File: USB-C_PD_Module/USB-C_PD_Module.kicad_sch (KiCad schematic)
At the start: 0 parts

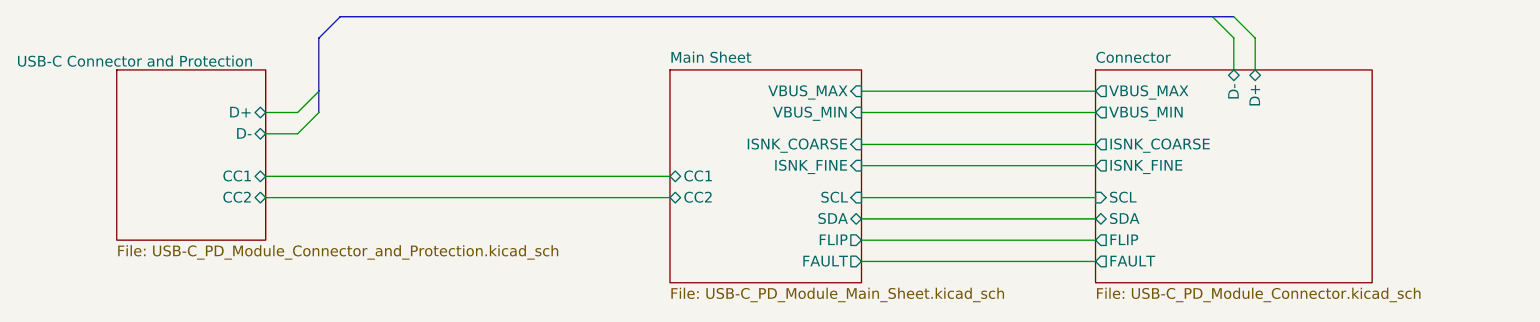
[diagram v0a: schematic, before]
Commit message: Module Basics
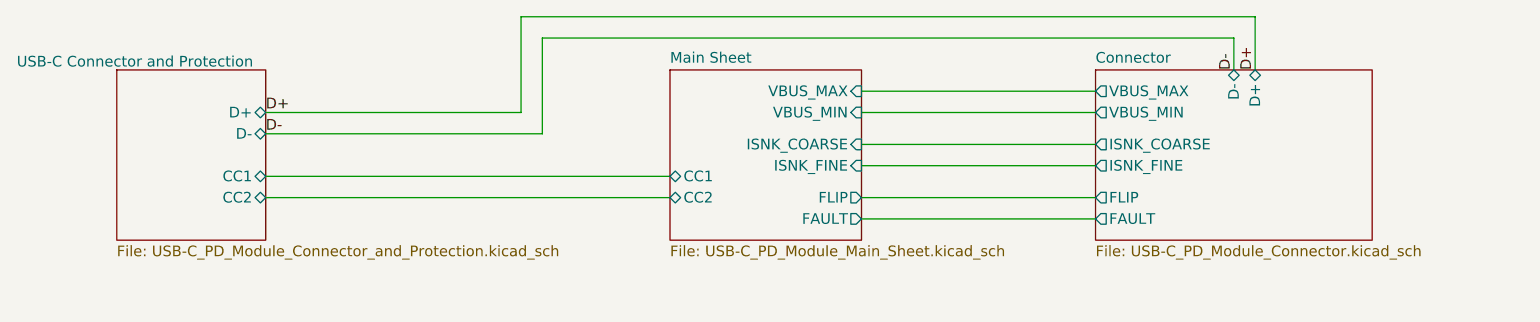
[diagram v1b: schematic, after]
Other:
- sheet Connector ports: added none; removed SCL, SDA
- sheet Main Sheet ports: added none; removed SCL, SDA
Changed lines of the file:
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@@
 		(rev "1.0")
 	)
-	(bus_entry
-		(at 210.82 88.9)
-		(size 2.54 2.54)
-		(stroke
-			(width 0)
-			(type default)
-		)
-	)
-	(bus_entry
-		(at 101.6 102.87)
-		(size 2.54 -2.54)
-		(stroke
-			(width 0)
-			(type default)
-		)
-	)
-	(bus_entry
-		(at 213.36 88.9)
-		(size 2.54 2.54)
-		(stroke
-			(width 0)
-			(type default)
-		)
-	)
-	(bus_entry
-		(at 101.6 100.33)
-		(size 2.54 -2.54)
-		(stroke
-			(width 0)
-			(type default)
-		)
-	)
 	(wire
 		(pts
@@
 	(wire
 		(pts
+			(xy 168.91 97.79) (xy 196.85 97.79)
+		)
+		(stroke
+			(width 0)
+			(type default)
+		)
+	)
+	(wire
+		(pts
+			(xy 215.9 88.9) (xy 215.9 95.25)
+		)
+		(stroke
+			(width 0)
+			(type default)
+		)
+	)
+	(wire
+		(pts
+			(xy 130.81 102.87) (xy 130.81 91.44)
+		)
+		(stroke
+			(width 0)
+			(type default)
+		)
+	)
+	(wire
+		(pts
+			(xy 168.91 106.68) (xy 196.85 106.68)
+		)
+		(stroke
+			(width 0)
+			(type default)
+		)
+	)
+	(wire
+		(pts
+			(xy 168.91 100.33) (xy 196.85 100.33)
+		)
+		(stroke
+			(width 0)
+			(type default)
+		)
+	)
+	(wire
+		(pts
+			(xy 128.27 88.9) (xy 215.9 88.9)
+		)
+		(stroke
+			(width 0)
+			(type default)
+		)
+	)
+	(wire
+		(pts
+			(xy 168.91 110.49) (xy 196.85 110.49)
+		)
+		(stroke
+			(width 0)
+			(type default)
+		)
+	)
+	(wire
+		(pts
 			(xy 168.91 113.03) (xy 196.85 113.03)
 		)
@@
 	(wire
 		(pts
-			(xy 168.91 97.79) (xy 196.85 97.79)
-		)
-		(stroke
-			(width 0)
-			(type default)
-		)
-	)
-	(wire
-		(pts
-			(xy 215.9 91.44) (xy 215.9 95.25)
-		)
-		(stroke
-			(width 0)
-			(type default)
-		)
-	)
-	(bus
-		(pts
-			(xy 104.14 91.44) (xy 106.68 88.9)
-		)
-		(stroke
-			(width 0)
-			(type default)
-		)
-	)
-	(wire
-		(pts
-			(xy 168.91 110.49) (xy 196.85 110.49)
-		)
-		(stroke
-			(width 0)
-			(type default)
-		)
-	)
-	(wire
-		(pts
-			(xy 168.91 106.68) (xy 196.85 106.68)
-		)
-		(stroke
-			(width 0)
-			(type default)
-		)
-	)
-	(wire
-		(pts
-			(xy 168.91 100.33) (xy 196.85 100.33)
-		)
-		(stroke
-			(width 0)
-			(type default)
-		)
-	)
-	(bus
-		(pts
-			(xy 104.14 97.79) (xy 104.14 100.33)
-		)
-		(stroke
-			(width 0)
-			(type default)
-		)
-	)
-	(wire
-		(pts
-			(xy 168.91 115.57) (xy 196.85 115.57)
-		)
-		(stroke
-			(width 0)
-			(type default)
-		)
-	)
-	(wire
-		(pts
-			(xy 168.91 118.11) (xy 196.85 118.11)
-		)
-		(stroke
-			(width 0)
-			(type default)
-		)
-	)
-	(bus
-		(pts
-			(xy 210.82 88.9) (xy 213.36 88.9)
-		)
-		(stroke
-			(width 0)
-			(type default)
-		)
-	)
-	(wire
-		(pts
 			(xy 97.79 107.95) (xy 146.05 107.95)
 		)
@@
 	(wire
 		(pts
-			(xy 97.79 102.87) (xy 101.6 102.87)
-		)
-		(stroke
-			(width 0)
-			(type default)
-		)
-	)
-	(wire
-		(pts
-			(xy 97.79 100.33) (xy 101.6 100.33)
-		)
-		(stroke
-			(width 0)
-			(type default)
-		)
-	)
-	(bus
-		(pts
-			(xy 104.14 91.44) (xy 104.14 97.79)
-		)
-		(stroke
-			(width 0)
-			(type default)
-		)
-	)
-	(bus
-		(pts
-			(xy 106.68 88.9) (xy 210.82 88.9)
+			(xy 97.79 102.87) (xy 130.81 102.87)
+		)
+		(stroke
+			(width 0)
+			(type default)
+		)
+	)
+	(wire
+		(pts
+			(xy 128.27 100.33) (xy 128.27 88.9)
+		)
+		(stroke
+			(width 0)
+			(type default)
+		)
+	)
+	(wire
+		(pts
+			(xy 97.79 100.33) (xy 128.27 100.33)
 		)
 		(stroke
@@
 			(width 0)
 			(type default)
+		)
+	)
+	(wire
+		(pts
+			(xy 130.81 91.44) (xy 213.36 91.44)
+		)
+		(stroke
+			(width 0)
+			(type default)
+		)
+	)
+	(label "D+"
+		(at 97.79 100.33 0)
+		(fields_autoplaced yes)
+		(effects
+			(font
+				(size 1.27 1.27)
+			)
+			(justify left bottom)
+		)
+	)
+	(label "D-"
+		(at 97.79 102.87 0)
+		(fields_autoplaced yes)
+		(effects
+			(font
+				(size 1.27 1.27)
+			)
+			(justify left bottom)
+		)
+	)
+	(label "D+"
+		(at 215.9 95.25 90)
+		(fields_autoplaced yes)
+		(effects
+			(font
+				(size 1.27 1.27)
+			)
+			(justify left bottom)
+		)
+	)
+	(label "D-"
+		(at 213.36 95.25 90)
+		(fields_autoplaced yes)
+		(effects
+			(font
+				(size 1.27 1.27)
+			)
+			(justify left bottom)
 		)
 	)
@@
 	(sheet
 		(at 196.85 95.25)
-		(size 33.02 25.4)
+		(size 33.02 20.32)
 		(fields_autoplaced yes)
 		(stroke
@@
 		)
 		(property "Sheetfile" "USB-C_PD_Module_Connector.kicad_sch"
-			(at 196.85 121.2346 0)
+			(at 196.85 116.1546 0)
 			(effects
 				(font
@@
 			)
 		)
-		(pin "SDA" bidirectional
+		(pin "FLIP" output
+			(at 196.85 110.49 180)
+			(effects
+				(font
+					(size 1.27 1.27)
+				)
+				(justify left)
+			)
+		)
+		(pin "FAULT" output
 			(at 196.85 113.03 180)
-			(effects
-				(font
-					(size 1.27 1.27)
-				)
-				(justify left)
-			)
-		)
-		(pin "SCL" input
-			(at 196.85 110.49 180)
-			(effects
-				(font
-					(size 1.27 1.27)
-				)
-				(justify left)
-			)
-		)
-		(pin "FLIP" output
-			(at 196.85 115.57 180)
-			(effects
-				(font
-					(size 1.27 1.27)
-				)
-				(justify left)
-			)
-		)
-		(pin "FAULT" output
-			(at 196.85 118.11 180)
 			(effects
 				(font
@@
 	(sheet
 		(at 146.05 95.25)
-		(size 22.86 25.4)
+		(size 22.86 20.32)
 		(fields_autoplaced yes)
 		(stroke
@@
 		)
 		(property "Sheetfile" "USB-C_PD_Module_Main_Sheet.kicad_sch"
-			(at 146.05 121.2346 0)
+			(at 146.05 116.1546 0)
 			(effects
 				(font
@@
 			)
 		)
-		(pin "SDA" bidirectional
+		(pin "FAULT" output
 			(at 168.91 113.03 0)
 			(effects
@@
 			)
 		)
-		(pin "FAULT" output
-			(at 168.91 118.11 0)
-			(effects
-				(font
-					(size 1.27 1.27)
-				)
-				(justify right)
-			)
-		)
 		(pin "FLIP" output
-			(at 168.91 115.57 0)
-			(effects
-				(font
-					(size 1.27 1.27)
-				)
-				(justify right)
-			)
-		)
-		(pin "SCL" input
 			(at 168.91 110.49 0)
 			(effects
